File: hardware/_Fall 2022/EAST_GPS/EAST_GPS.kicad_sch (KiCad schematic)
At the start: 2 parts, among them J1 Conn_02x10_Counter_Clockwise, U1 GPS-14414

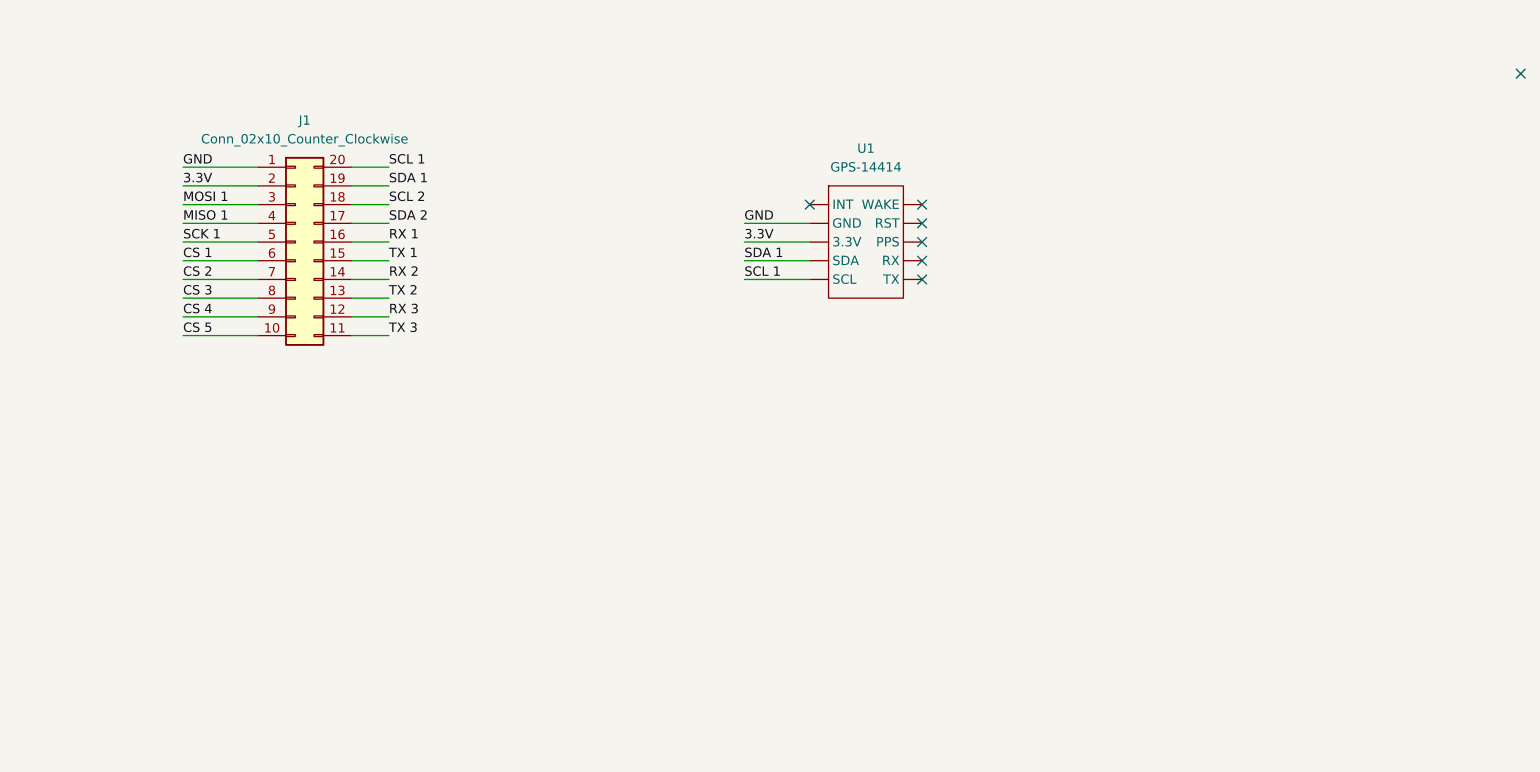
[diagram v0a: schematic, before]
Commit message: Update east communication and layout
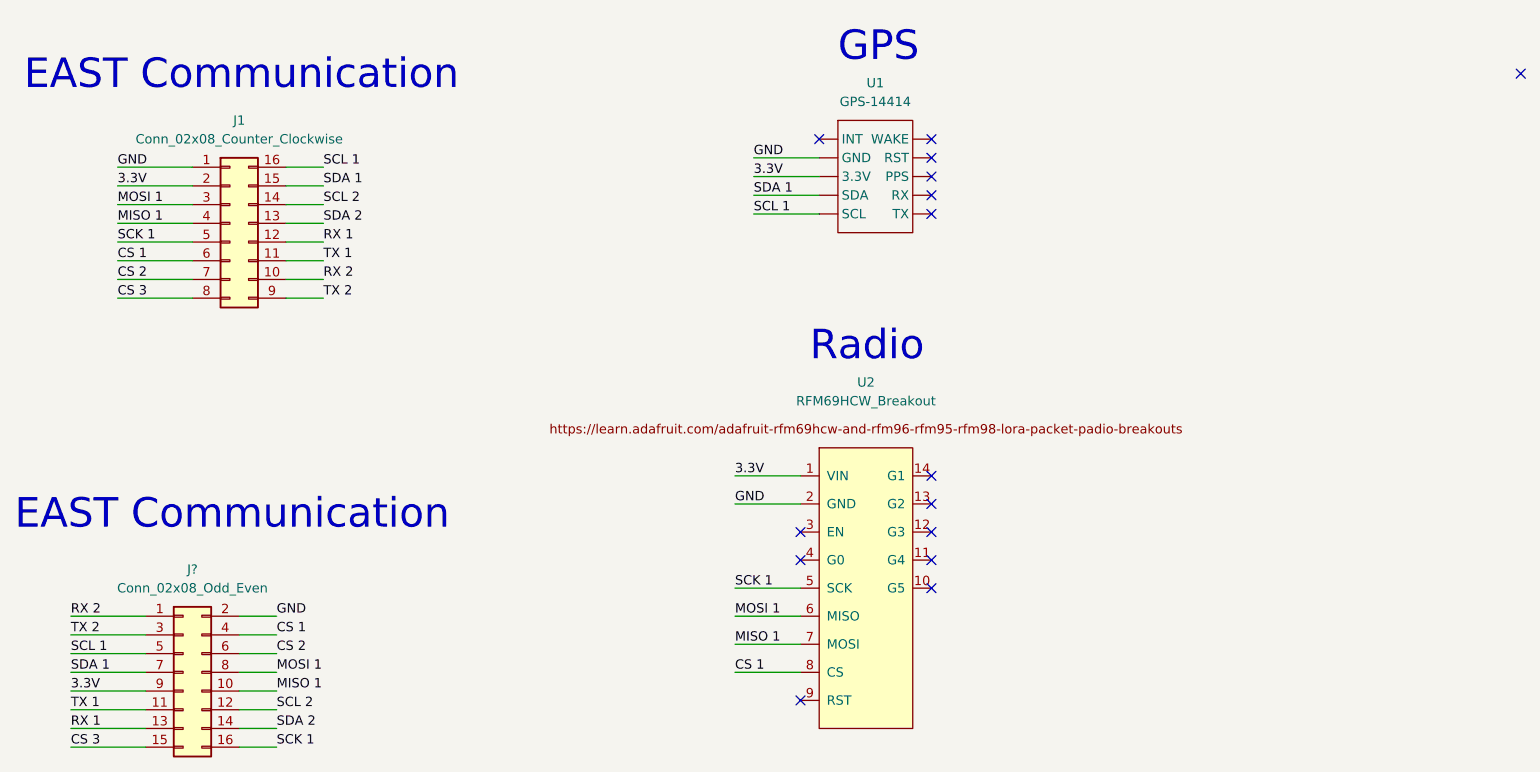
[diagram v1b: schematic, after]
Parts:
- removed J1: Conn_02x10_Counter_Clockwise, Connector_PinHeader_2.54mm:PinHeader_2x10_P2.54mm_Vertical, symbol Connector_Generic:Conn_02x10_Counter_Clockwise
- added J1: Conn_02x08_Counter_Clockwise, Connector_PinHeader_2.54mm:PinHeader_2x08_P2.54mm_Vertical, symbol Connector_Generic:Conn_02x08_Counter_Clockwise
- added J?: Conn_02x08_Odd_Even, Connector_PinHeader_2.54mm:PinHeader_2x08_P2.54mm_Vertical, symbol Connector_Generic:Conn_02x08_Odd_Even
- added U2: RFM69HCW_Breakout, Sensors:RFM69HCW_Breakout, symbol sensors:RFM69HCW_Breakout
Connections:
- net 3.3V: now also J1.2 (Pin_2), J?.9 (Pin_9), U2.1 (VIN)
- net CS 1: now also J1.6 (Pin_6), J?.4 (Pin_4), U2.8 (CS)
- net CS 2: now also J1.7 (Pin_7), J?.6 (Pin_6)
- net CS 3: now also J1.8 (Pin_8), J?.15 (Pin_15)
- net GND: now also J1.1 (Pin_1), J?.2 (Pin_2), U2.2 (GND)
- net MISO 1: now also J1.4 (Pin_4), J?.10 (Pin_10), U2.7 (MOSI)
- net MOSI 1: now also J1.3 (Pin_3), J?.8 (Pin_8), U2.6 (MISO)
- net RX 1: now also J1.12 (Pin_12), J?.13 (Pin_13)
- net RX 2: now also J1.10 (Pin_10), J?.1 (Pin_1)
- net SCK 1: now also J1.5 (Pin_5), J?.16 (Pin_16), U2.5 (SCK)
- net SCL 1: now also J1.16 (Pin_16), J?.5 (Pin_5)
- net SCL 2: now also J1.14 (Pin_14), J?.12 (Pin_12)
- net SDA 1: now also J1.15 (Pin_15), J?.7 (Pin_7)
- net SDA 2: now also J1.13 (Pin_13), J?.14 (Pin_14)
- net TX 1: now also J1.11 (Pin_11), J?.11 (Pin_11)
- net TX 2: now also J1.9 (Pin_9), J?.3 (Pin_3)
- no-connect marks 7 -> 15
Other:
- note added: "EAST Communication"
- note added: "GPS"
- note added: "Radio"
- moved on the sheet: U1
